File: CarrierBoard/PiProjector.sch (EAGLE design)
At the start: 73 parts, among them P8 PINHEAD2X23, P9 PINHEAD2X23, X1 24MHz, X2 12Mhz

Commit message: POE connection Moved
Started Modification for Adjusted POE connection
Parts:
- removed AUX_BTN: (no value), pinhead:PINHD-2X4
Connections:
- removed net MUTEP: AUX_BTN.4, U$6.MUTEP
- removed net MUTEREC: AUX_BTN.8, U$6.MUTER
- removed net VOLDN: AUX_BTN.6, U$6.VOLDN
- removed net VOLUP: AUX_BTN.2, U$6.VOLUP
- new net MUTP: P8.7, U$6.MUTEP
- new net MUTR: P8.8, U$6.MUTER
- new net VLDN: P8.10, U$6.VOLDN
- new net VLUP: P8.9, U$6.VOLUP
- net +5V: now also P8.3, P8.4; no longer AUX_BTN.5
- net GND: now also P8.1, P8.2; no longer AUX_BTN.7
- net POE+: now also P8.5; no longer AUX_BTN.1
- net POE-: now also P8.6; no longer AUX_BTN.3
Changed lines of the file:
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@@
 <part name="SUPPLY20" library="supply2" library_urn="urn:adsk.eagle:library:372" deviceset="GND" device=""/>
 <part name="SUPPLY17" library="supply2" library_urn="urn:adsk.eagle:library:372" deviceset="GND" device=""/>
-<part name="AUX_BTN" library="pinhead" library_urn="urn:adsk.eagle:library:325" deviceset="PINHD-2X4" device="" package3d_urn="urn:adsk.eagle:package:22461/2"/>
-<part name="SUPPLY22" library="supply2" library_urn="urn:adsk.eagle:library:372" deviceset="GND" device=""/>
 <part name="U$7" library="PiProject" deviceset="SJ-43514-SMT-TR" device=""/>
 <part name="C16" library="pm-labs" deviceset="C" device="1206DR" value="100u">
@@
 <part name="R16" library="pm-labs" deviceset="R" device="0603R" value="5.1K"/>
 <part name="SUPPLY28" library="supply2" library_urn="urn:adsk.eagle:library:372" deviceset="GND" device=""/>
+<part name="SUPPLY29" library="supply2" library_urn="urn:adsk.eagle:library:372" deviceset="GND" device=""/>
+<part name="SUPPLY30" library="supply2" library_urn="urn:adsk.eagle:library:372" deviceset="GND" device=""/>
 </parts>
 <sheets>
@@
 <attribute name="VALUE" x="401.955" y="146.685" size="1.778" layer="96"/>
 </instance>
-<instance part="AUX_BTN" gate="A" x="363.22" y="162.56" smashed="yes" rot="R180">
-<attribute name="NAME" x="369.57" y="169.545" size="1.778" layer="95" rot="R180"/>
-<attribute name="VALUE" x="369.57" y="170.18" size="1.778" layer="96" rot="R180"/>
-</instance>
-<instance part="SUPPLY22" gate="GND" x="368.3" y="149.86" smashed="yes">
-<attribute name="VALUE" x="366.395" y="146.685" size="1.778" layer="96"/>
-</instance>
 <instance part="U$7" gate="G$1" x="439.42" y="215.9" smashed="yes" rot="R270"/>
 <instance part="C16" gate="G$1" x="424.18" y="233.68" smashed="yes" rot="R90">
@@
 <instance part="SUPPLY28" gate="GND" x="271.78" y="137.16" smashed="yes">
 <attribute name="VALUE" x="269.875" y="133.985" size="1.778" layer="96"/>
+</instance>
+<instance part="SUPPLY29" gate="GND" x="0" y="213.36" smashed="yes">
+<attribute name="VALUE" x="-1.905" y="210.185" size="1.778" layer="96"/>
+</instance>
+<instance part="SUPPLY30" gate="GND" x="-43.18" y="213.36" smashed="yes">
+<attribute name="VALUE" x="-45.085" y="210.185" size="1.778" layer="96"/>
 </instance>
 </instances>
@@
 </segment>
 <segment>
-<pinref part="AUX_BTN" gate="A" pin="7"/>
-<wire x1="365.76" y1="165.1" x2="368.3" y2="165.1" width="0.1524" layer="91"/>
-<wire x1="368.3" y1="165.1" x2="368.3" y2="152.4" width="0.1524" layer="91"/>
-<pinref part="SUPPLY22" gate="GND" pin="GND"/>
-</segment>
-<segment>
 <pinref part="C19" gate="G$1" pin="2"/>
 <wire x1="419.1" y1="238.76" x2="449.58" y2="238.76" width="0.1524" layer="91"/>
@@
 <pinref part="SUPPLY28" gate="GND" pin="GND"/>
 <junction x="271.78" y="139.7"/>
+</segment>
+<segment>
+<pinref part="P8" gate="G$1" pin="2"/>
+<wire x1="-17.78" y1="215.9" x2="0" y2="215.9" width="0.1524" layer="91"/>
+<pinref part="SUPPLY29" gate="GND" pin="GND"/>
+</segment>
+<segment>
+<pinref part="P8" gate="G$1" pin="1"/>
+<wire x1="-25.4" y1="215.9" x2="-43.18" y2="215.9" width="0.1524" layer="91"/>
+<pinref part="SUPPLY30" gate="GND" pin="GND"/>
 </segment>
 </net>
@@
 </segment>
 <segment>
-<pinref part="AUX_BTN" gate="A" pin="5"/>
-<wire x1="365.76" y1="162.56" x2="373.38" y2="162.56" width="0.1524" layer="91"/>
-<label x="370.84" y="162.56" size="1.778" layer="95"/>
+<pinref part="P8" gate="G$1" pin="3"/>
+<wire x1="-25.4" y1="213.36" x2="-38.1" y2="213.36" width="0.1524" layer="91"/>
+<label x="-38.1" y="213.36" size="1.778" layer="95"/>
+</segment>
+<segment>
+<pinref part="P8" gate="G$1" pin="4"/>
+<wire x1="-17.78" y1="213.36" x2="-5.08" y2="213.36" width="0.1524" layer="91"/>
+<label x="-10.16" y="213.36" size="1.778" layer="95"/>
 </segment>
 </net>
@@
 </segment>
 </net>
-<net name="MUTEREC" class="0">
-<segment>
-<pinref part="U$6" gate="G$1" pin="MUTER"/>
-<wire x1="393.7" y1="180.34" x2="393.7" y2="165.1" width="0.1524" layer="91"/>
-<label x="393.7" y="165.1" size="1.778" layer="95" rot="R90"/>
-</segment>
-<segment>
-<pinref part="AUX_BTN" gate="A" pin="8"/>
-<wire x1="358.14" y1="165.1" x2="350.52" y2="165.1" width="0.1524" layer="91"/>
-<label x="347.98" y="165.1" size="1.778" layer="95"/>
-</segment>
-</net>
 <net name="USB2D_P" class="1">
 <segment>
@@
 <pinref part="C17" gate="G$1" pin="2"/>
 <pinref part="U$7" gate="G$1" pin="LEFT"/>
-</segment>
-</net>
-<net name="MUTEP" class="0">
-<segment>
-<label x="347.98" y="160.02" size="1.778" layer="95"/>
-<pinref part="AUX_BTN" gate="A" pin="4"/>
-<wire x1="350.52" y1="160.02" x2="358.14" y2="160.02" width="0.1524" layer="91"/>
-</segment>
-<segment>
-<pinref part="U$6" gate="G$1" pin="MUTEP"/>
-<wire x1="419.1" y1="203.2" x2="426.72" y2="203.2" width="0.1524" layer="91"/>
-<label x="426.72" y="203.2" size="1.778" layer="95" rot="R90"/>
-<wire x1="426.72" y1="203.2" x2="426.72" y2="210.82" width="0.1524" layer="91"/>
-</segment>
-</net>
-<net name="VOLDN" class="0">
-<segment>
-<label x="347.98" y="162.56" size="1.778" layer="95"/>
-<pinref part="AUX_BTN" gate="A" pin="6"/>
-<wire x1="358.14" y1="162.56" x2="350.52" y2="162.56" width="0.1524" layer="91"/>
-</segment>
-<segment>
-<pinref part="U$6" gate="G$1" pin="VOLDN"/>
-<wire x1="370.84" y1="190.5" x2="363.22" y2="190.5" width="0.1524" layer="91"/>
-<label x="363.22" y="187.96" size="1.778" layer="95"/>
-</segment>
-</net>
-<net name="VOLUP" class="0">
-<segment>
-<pinref part="AUX_BTN" gate="A" pin="2"/>
-<wire x1="358.14" y1="157.48" x2="350.52" y2="157.48" width="0.1524" layer="91"/>
-<label x="347.98" y="157.48" size="1.778" layer="95"/>
-</segment>
-<segment>
-<pinref part="U$6" gate="G$1" pin="VOLUP"/>
-<wire x1="370.84" y1="213.36" x2="350.52" y2="213.36" width="0.1524" layer="91"/>
-<label x="350.52" y="213.36" size="1.778" layer="95"/>
 </segment>
 </net>
@@
 </segment>
 <segment>
-<pinref part="AUX_BTN" gate="A" pin="1"/>
-<wire x1="365.76" y1="157.48" x2="381" y2="157.48" width="0.1524" layer="91"/>
-<label x="373.38" y="157.48" size="1.778" layer="95"/>
+<pinref part="P8" gate="G$1" pin="5"/>
+<wire x1="-38.1" y1="210.82" x2="-25.4" y2="210.82" width="0.1524" layer="91"/>
+<label x="-38.1" y="210.82" size="1.778" layer="95"/>
 </segment>
 </net>
@@
 </segment>
 <segment>
-<pinref part="AUX_BTN" gate="A" pin="3"/>
-<wire x1="381" y1="160.02" x2="365.76" y2="160.02" width="0.1524" layer="91"/>
-<label x="373.38" y="160.02" size="1.778" layer="95"/>
+<pinref part="P8" gate="G$1" pin="6"/>
+<wire x1="-17.78" y1="210.82" x2="-7.62" y2="210.82" width="0.1524" layer="91"/>
+<wire x1="-5.08" y1="210.82" x2="-7.62" y2="210.82" width="0.1524" layer="91"/>
+<label x="-10.16" y="210.82" size="1.778" layer="95"/>
 </segment>
 </net>
@@
 </segment>
 </net>
+<net name="MUTP" class="0">
+<segment>
+<pinref part="P8" gate="G$1" pin="7"/>
+<wire x1="-25.4" y1="208.28" x2="-38.1" y2="208.28" width="0.1524" layer="91"/>
+<label x="-38.1" y="208.28" size="1.778" layer="95"/>
+</segment>
+<segment>
+<pinref part="U$6" gate="G$1" pin="MUTEP"/>
+<wire x1="419.1" y1="203.2" x2="426.72" y2="203.2" width="0.1524" layer="91"/>
+<label x="426.72" y="203.2" size="1.778" layer="95" rot="R90"/>
+<wire x1="426.72" y1="203.2" x2="426.72" y2="210.82" width="0.1524" layer="91"/>
+</segment>
+</net>
+<net name="VLUP" class="0">
+<segment>
+<pinref part="P8" gate="G$1" pin="9"/>
+<wire x1="-25.4" y1="205.74" x2="-38.1" y2="205.74" width="0.1524" layer="91"/>
+<label x="-38.1" y="205.74" size="1.778" layer="95"/>
+</segment>
+<segment>
+<pinref part="U$6" gate="G$1" pin="VOLUP"/>
+<wire x1="370.84" y1="213.36" x2="350.52" y2="213.36" width="0.1524" layer="91"/>
+<label x="350.52" y="213.36" size="1.778" layer="95"/>
+</segment>
+</net>
+<net name="MUTR" class="0">
+<segment>
+<pinref part="P8" gate="G$1" pin="8"/>
+<wire x1="-17.78" y1="208.28" x2="-5.08" y2="208.28" width="0.1524" layer="91"/>
+<label x="-12.7" y="208.28" size="1.778" layer="95"/>
+</segment>
+<segment>
+<pinref part="U$6" gate="G$1" pin="MUTER"/>
+<wire x1="393.7" y1="180.34" x2="393.7" y2="165.1" width="0.1524" layer="91"/>
+<label x="393.7" y="165.1" size="1.778" layer="95" rot="R90"/>
+</segment>
+</net>
+<net name="VLDN" class="0">
+<segment>
+<pinref part="P8" gate="G$1" pin="10"/>
+<wire x1="-17.78" y1="205.74" x2="-5.08" y2="205.74" width="0.1524" layer="91"/>
+<label x="-12.7" y="205.74" size="1.778" layer="95"/>
+</segment>
+<segment>
+<pinref part="U$6" gate="G$1" pin="VOLDN"/>
+<wire x1="370.84" y1="190.5" x2="363.22" y2="190.5" width="0.1524" layer="91"/>
+<label x="363.22" y="187.96" size="1.778" layer="95"/>
+</segment>
+</net>

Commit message: Testing nRPIBOOT fix
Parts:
- removed !RPI_BOOT: TP1R, pm-labs:TP1R
- added Q1, Q2: BCX70SMD, transistor-npn:BCX70SMD
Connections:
- removed net N$25: R2.1, R8.1, RPI-CM1G$2.USB_OTG_ID, SLAVE_SWITCH.2, U$1.SEL
- removed net N$36: !RPI_BOOT.1, RPI-CM1G$1.!RPIBOOT
- new net !RPIBOOT: Q2.C, RPI-CM1G$1.!RPIBOOT
- new net N$2: LED1.C, Q1.C, R2.2
- new net N$7: Q1.E, Q2.E, SLAVE_SWITCH.2
- new net SELECT: R2.1, R8.1, RPI-CM1G$2.USB_OTG_ID, U$1.SEL
- net +3.3V: now also Q1.B, Q2.B; no longer SLAVE_SWITCH.1
- net GND: now also SLAVE_SWITCH.1; no longer LED1.C, R2.2
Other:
- moved on the sheet: R2, SLAVE_SWITCH

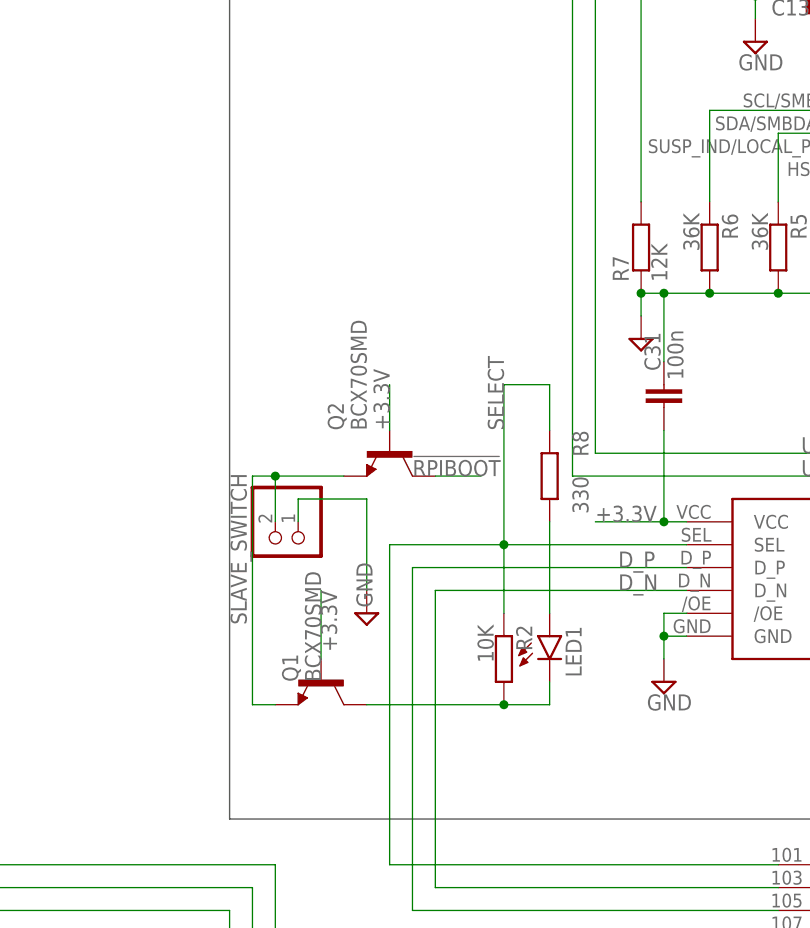
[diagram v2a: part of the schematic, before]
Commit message: Need PM labs
replace transistor with pfet and diode with shotkey diode
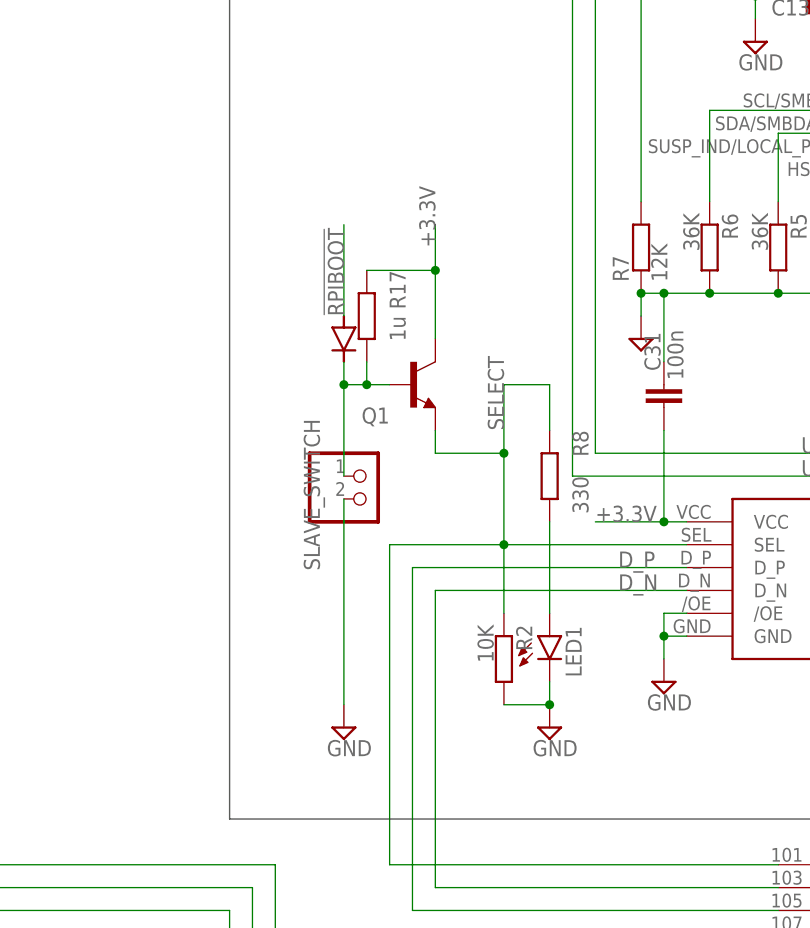
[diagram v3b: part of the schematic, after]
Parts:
- removed Q2: BCX70SMD, transistor-npn:BCX70SMD
- added R17: 1u, pm-labs:R0603R
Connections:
- removed net N$2: LED1.C, Q1.C, R2.2
- removed net N$7: Q1.E, Q2.E, SLAVE_SWITCH.2
- new net N$8: Q1.B, R17.2, SLAVE_SWITCH.1
- net !RPIBOOT: no longer Q2.C
- net +3.3V: now also Q1.C, R17.1; no longer Q1.B, Q2.B
- net GND: now also LED1.C, R2.2, SLAVE_SWITCH.2; no longer SLAVE_SWITCH.1
- net SELECT: now also Q1.E
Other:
- moved on the sheet: Q1, SLAVE_SWITCH
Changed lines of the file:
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@@
 <part name="SUPPLY30" library="supply2" library_urn="urn:adsk.eagle:library:372" deviceset="GND" device=""/>
 <part name="Q1" library="transistor-npn" library_urn="urn:adsk.eagle:library:398" deviceset="BCX70*" device="SMD" package3d_urn="urn:adsk.eagle:package:28738/2"/>
-<part name="Q2" library="transistor-npn" library_urn="urn:adsk.eagle:library:398" deviceset="BCX70*" device="SMD" package3d_urn="urn:adsk.eagle:package:28738/2"/>
+<part name="R17" library="pm-labs" deviceset="R" device="0603R" value="1u"/>
 <part name="SUPPLY5" library="supply2" library_urn="urn:adsk.eagle:library:372" deviceset="GND" device=""/>
+<part name="SUPPLY22" library="supply2" library_urn="urn:adsk.eagle:library:372" deviceset="GND" device=""/>
+<part name="D3" library="docu-dummy" library_urn="urn:adsk.eagle:library:215" deviceset="DIODE" device=""/>
 </parts>
 <sheets>
@@
 <attribute name="NOTE" x="414.02" y="231.14" size="1.778" layer="96" rot="R90" display="off"/>
 </instance>
-<instance part="SLAVE_SWITCH" gate="G$1" x="132.08" y="177.8" smashed="yes" rot="R270">
-<attribute name="NAME" x="128.905" y="168.91" size="1.778" layer="95" rot="R90"/>
-<attribute name="VALUE" x="127" y="184.15" size="1.778" layer="96" rot="R270"/>
+<instance part="SLAVE_SWITCH" gate="G$1" x="142.24" y="182.88" smashed="yes">
+<attribute name="NAME" x="135.255" y="191.77" size="1.778" layer="95" rot="R270"/>
+<attribute name="VALUE" x="135.89" y="177.8" size="1.778" layer="96"/>
 </instance>
 <instance part="C18" gate="G$1" x="431.8" y="236.22" smashed="yes" rot="R90">
@@
 <attribute name="VALUE" x="-45.085" y="210.185" size="1.778" layer="96"/>
 </instance>
-<instance part="Q1" gate="G$1" x="137.16" y="162.56" smashed="yes" rot="R270">
-<attribute name="NAME" x="134.62" y="162.56" size="1.778" layer="95" rot="R90"/>
-<attribute name="VALUE" x="137.16" y="162.56" size="1.778" layer="96" rot="R90"/>
-</instance>
-<instance part="Q2" gate="G$1" x="144.78" y="187.96" smashed="yes" rot="R270">
-<attribute name="NAME" x="139.7" y="190.5" size="1.778" layer="95" rot="R90"/>
-<attribute name="VALUE" x="142.24" y="190.5" size="1.778" layer="96" rot="R90"/>
-</instance>
-<instance part="SUPPLY5" gate="GND" x="142.24" y="170.18" smashed="yes">
-<attribute name="VALUE" x="142.875" y="170.815" size="1.778" layer="96" rot="R90"/>
-</instance>
+<instance part="Q1" gate="G$1" x="147.32" y="195.58" smashed="yes">
+<attribute name="NAME" x="144.78" y="193.04" size="1.778" layer="95" rot="R180"/>
+</instance>
+<instance part="R17" gate="R" x="142.24" y="203.2" smashed="yes" rot="R270">
+<attribute name="NAME" x="144.78" y="208.28" size="1.778" layer="95" rot="R270"/>
+<attribute name="VALUE" x="144.78" y="203.2" size="1.778" layer="96" rot="R270"/>
+</instance>
+<instance part="SUPPLY5" gate="GND" x="162.56" y="157.48" smashed="yes">
+<attribute name="VALUE" x="160.655" y="154.305" size="1.778" layer="96"/>
+</instance>
+<instance part="SUPPLY22" gate="GND" x="139.7" y="157.48" smashed="yes">
+<attribute name="VALUE" x="137.795" y="154.305" size="1.778" layer="96"/>
+</instance>
+<instance part="D3" gate="G$1" x="139.7" y="200.66" smashed="yes" rot="R270"/>
 </instances>
 <busses>
@@
 </segment>
 <segment>
-<pinref part="SLAVE_SWITCH" gate="G$1" pin="1"/>
-<wire x1="134.62" y1="180.34" x2="134.62" y2="182.88" width="0.1524" layer="91"/>
-<wire x1="134.62" y1="182.88" x2="142.24" y2="182.88" width="0.1524" layer="91"/>
-<wire x1="142.24" y1="182.88" x2="142.24" y2="172.72" width="0.1524" layer="91"/>
+<wire x1="162.56" y1="162.56" x2="162.56" y2="160.02" width="0.1524" layer="91"/>
+<pinref part="LED1" gate="G$1" pin="C"/>
+<pinref part="R2" gate="R" pin="2"/>
+<wire x1="162.56" y1="160.02" x2="157.48" y2="160.02" width="0.1524" layer="91"/>
 <pinref part="SUPPLY5" gate="GND" pin="GND"/>
+<junction x="162.56" y="160.02"/>
+</segment>
+<segment>
+<pinref part="SLAVE_SWITCH" gate="G$1" pin="2"/>
+<wire x1="139.7" y1="182.88" x2="139.7" y2="160.02" width="0.1524" layer="91"/>
+<pinref part="SUPPLY22" gate="GND" pin="GND"/>
 </segment>
 </net>
@@
 </segment>
 <segment>
-<pinref part="Q1" gate="G$1" pin="B"/>
-<wire x1="137.16" y1="165.1" x2="137.16" y2="172.72" width="0.1524" layer="91"/>
-<label x="137.16" y="172.72" size="1.778" layer="95" rot="R270"/>
-</segment>
-<segment>
-<pinref part="Q2" gate="G$1" pin="B"/>
-<wire x1="144.78" y1="190.5" x2="144.78" y2="195.58" width="0.1524" layer="91"/>
-<label x="144.78" y="190.5" size="1.778" layer="95" rot="R90"/>
+<pinref part="Q1" gate="G$1" pin="C"/>
+<wire x1="149.86" y1="208.28" x2="149.86" y2="200.66" width="0.1524" layer="91"/>
+<pinref part="R17" gate="R" pin="1"/>
+<wire x1="149.86" y1="208.28" x2="142.24" y2="208.28" width="0.1524" layer="91"/>
+<junction x="149.86" y="208.28"/>
+<wire x1="149.86" y1="213.36" x2="149.86" y2="208.28" width="0.1524" layer="91"/>
+<label x="149.86" y="210.82" size="1.778" layer="95" rot="R90"/>
 </segment>
 </net>
@@
 </segment>
 <segment>
-<pinref part="Q2" gate="G$1" pin="C"/>
-<wire x1="149.86" y1="185.42" x2="154.94" y2="185.42" width="0.1524" layer="91"/>
-<label x="147.32" y="185.42" size="1.778" layer="95"/>
+<wire x1="139.7" y1="203.2" x2="139.7" y2="213.36" width="0.1524" layer="91"/>
+<label x="139.7" y="203.2" size="1.778" layer="95" rot="R90"/>
 </segment>
 </net>
@@
 <wire x1="370.84" y1="190.5" x2="363.22" y2="190.5" width="0.1524" layer="91"/>
 <label x="363.22" y="187.96" size="1.778" layer="95"/>
-</segment>
-</net>
-<net name="N$2" class="3">
-<segment>
-<wire x1="162.56" y1="162.56" x2="162.56" y2="160.02" width="0.1524" layer="91"/>
-<pinref part="LED1" gate="G$1" pin="C"/>
-<pinref part="R2" gate="R" pin="2"/>
-<pinref part="Q1" gate="G$1" pin="C"/>
-<wire x1="157.48" y1="160.02" x2="142.24" y2="160.02" width="0.1524" layer="91"/>
-<wire x1="162.56" y1="160.02" x2="157.48" y2="160.02" width="0.1524" layer="91"/>
-<junction x="157.48" y="160.02"/>
-</segment>
-</net>
-<net name="N$7" class="0">
-<segment>
-<pinref part="SLAVE_SWITCH" gate="G$1" pin="2"/>
-<pinref part="Q2" gate="G$1" pin="E"/>
-<wire x1="139.7" y1="185.42" x2="132.08" y2="185.42" width="0.1524" layer="91"/>
-<wire x1="132.08" y1="185.42" x2="129.54" y2="185.42" width="0.1524" layer="91"/>
-<wire x1="129.54" y1="185.42" x2="129.54" y2="160.02" width="0.1524" layer="91"/>
-<pinref part="Q1" gate="G$1" pin="E"/>
-<wire x1="129.54" y1="160.02" x2="132.08" y2="160.02" width="0.1524" layer="91"/>
-<wire x1="132.08" y1="180.34" x2="132.08" y2="185.42" width="0.1524" layer="91"/>
-<junction x="132.08" y="185.42"/>
 </segment>
 </net>
@@
 <wire x1="162.56" y1="195.58" x2="162.56" y2="190.5" width="0.1524" layer="91"/>
 <wire x1="157.48" y1="195.58" x2="162.56" y2="195.58" width="0.1524" layer="91"/>
-<wire x1="157.48" y1="195.58" x2="157.48" y2="177.8" width="0.1524" layer="91"/>
+<wire x1="157.48" y1="195.58" x2="157.48" y2="187.96" width="0.1524" layer="91"/>
 <label x="157.48" y="190.5" size="1.778" layer="95" rot="R90"/>
-</segment>
-</net>
+<pinref part="Q1" gate="G$1" pin="E"/>
+<wire x1="157.48" y1="187.96" x2="157.48" y2="177.8" width="0.1524" layer="91"/>
+<wire x1="149.86" y1="190.5" x2="149.86" y2="187.96" width="0.1524" layer="91"/>
+<wire x1="149.86" y1="187.96" x2="157.48" y2="187.96" width="0.1524" layer="91"/>
+<junction x="157.48" y="187.96"/>
+</segment>
+</net>
+<net name="N$8" class="0">
+<segment>
+<pinref part="R17" gate="R" pin="2"/>
+<wire x1="142.24" y1="198.12" x2="142.24" y2="195.58" width="0.1524" layer="91"/>
+<pinref part="Q1" gate="G$1" pin="B"/>
+<wire x1="142.24" y1="195.58" x2="144.78" y2="195.58" width="0.1524" layer="91"/>
+<wire x1="142.24" y1="195.58" x2="139.7" y2="195.58" width="0.1524" layer="91"/>
+<wire x1="139.7" y1="195.58" x2="139.7" y2="185.42" width="0.1524" layer="91"/>
+<junction x="142.24" y="195.58"/>
+<pinref part="SLAVE_SWITCH" gate="G$1" pin="1"/>
+<wire x1="139.7" y1="195.58" x2="139.7" y2="198.12" width="0.1524" layer="91"/>
+<junction x="139.7" y="195.58"/>
+</segment>
+</net>
